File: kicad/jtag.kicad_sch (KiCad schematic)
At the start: 50 parts, among them J3 USB4105-GF-A, J4 Conn_01x02_Male, J5 3220-10-0100-00, U10 NTB0104BQ,115, U13 NTB0104BQ,115, U17 93C56, U2 FT2232HL-REEL, Y2 12MHz

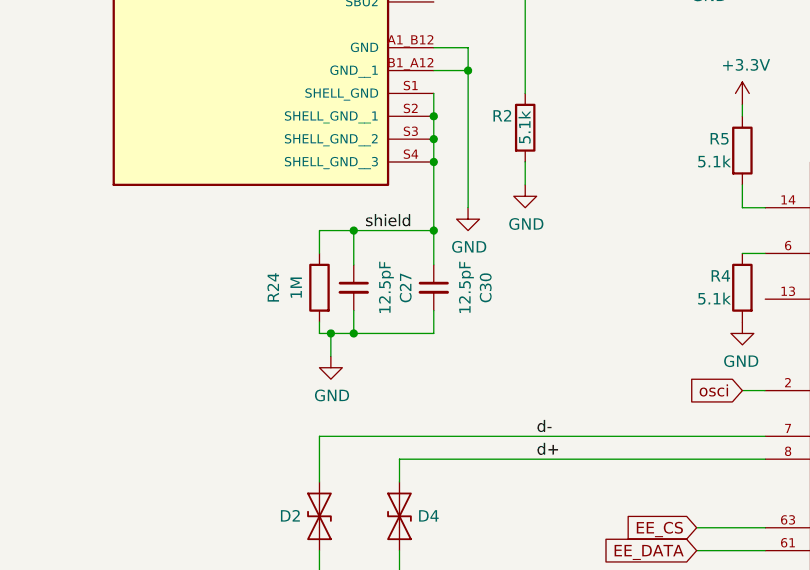
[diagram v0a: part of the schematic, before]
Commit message: directly grounded the USB shield
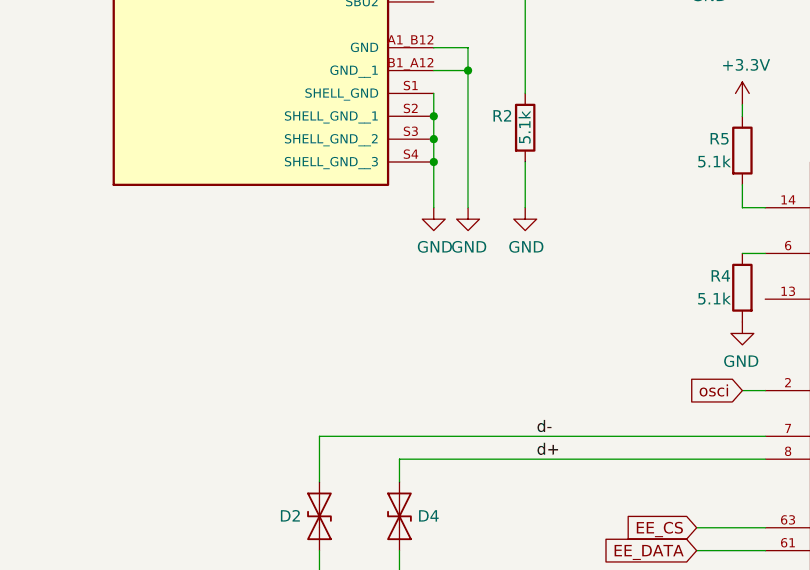
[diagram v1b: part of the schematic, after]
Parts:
- removed C27, C30: 12.5pF, Capacitor_SMD:C_0603_1608Metric, symbol Device:C_Small
- removed R24: 1M, Resistor_SMD:R_0603_1608Metric_Pad0.98x0.95mm_HandSolder, symbol Device:R
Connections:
- net shield is gone; now on net GND: J3.S1 (SHELL_GND), J3.S2 (SHELL_GND__1), J3.S3 (SHELL_GND__2), J3.S4 (SHELL_GND__3)
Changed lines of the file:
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@@
 (kicad_sch (version 20230121) (generator eeschema)
   (paper "A4")
-  (junction (at 62.23 76.2) (diameter 0) (color 0 0 0 0)
-  )
   (junction (at 255.27 67.31) (diameter 0) (color 0 0 0 0)
   )
   (junction (at 250.19 62.23) (diameter 0) (color 0 0 0 0)
   )
-  (junction (at 62.23 64.77) (diameter 0) (color 0 0 0 0)
-  )
   (junction (at 140.97 25.4) (diameter 0) (color 0 0 0 0)
   )
@@
   (junction (at 245.11 115.57) (diameter 0) (color 0 0 0 0)
   )
-  (junction (at 71.12 64.77) (diameter 0) (color 0 0 0 0)
-  )
   (junction (at 166.37 77.47) (diameter 0) (color 0 0 0 0)
   )
@@
   (junction (at 242.57 57.15) (diameter 0) (color 0 0 0 0)
   )
-  (junction (at 59.69 76.2) (diameter 0) (color 0 0 0 0)
-  )
   (junction (at 22.86 185.42) (diameter 0) (color 0 0 0 0)
   )
@@
     (stroke (width 0) (type default))
   )
-  (wire (pts (xy 71.12 68.58) (xy 71.12 64.77))
-    (stroke (width 0) (type default))
-  )
   (wire (pts (xy 200.66 34.29) (xy 190.5 34.29))
     (stroke (width 0) (type default))
@@
     (stroke (width 0) (type default))
   )
-  (wire (pts (xy 59.69 76.2) (xy 59.69 78.74))
+  (wire (pts (xy 71.12 57.15) (xy 71.12 62.23))
     (stroke (width 0) (type default))
   )
@@
     (stroke (width 0) (type default))
   )
-  (wire (pts (xy 71.12 57.15) (xy 71.12 64.77))
-    (stroke (width 0) (type default))
-  )
   (wire (pts (xy 163.83 67.31) (xy 185.42 67.31))
     (stroke (width 0) (type default))
@@
     (stroke (width 0) (type default))
   )
-  (wire (pts (xy 71.12 73.66) (xy 71.12 76.2))
-    (stroke (width 0) (type default))
-  )
   (wire (pts (xy 163.83 62.23) (xy 163.83 64.77))
     (stroke (width 0) (type default))
@@
     (stroke (width 0) (type default))
   )
-  (wire (pts (xy 58.42 67.31) (xy 58.42 64.77))
-    (stroke (width 0) (type default))
-  )
   (wire (pts (xy 158.75 92.71) (xy 185.42 92.71))
     (stroke (width 0) (type default))
@@
     (stroke (width 0) (type default))
   )
-  (wire (pts (xy 62.23 64.77) (xy 71.12 64.77))
-    (stroke (width 0) (type default))
-  )
   (wire (pts (xy 105.41 120.65) (xy 105.41 118.11))
     (stroke (width 0) (type default))
@@
     (stroke (width 0) (type default))
   )
-  (wire (pts (xy 81.28 59.69) (xy 81.28 57.15))
+  (wire (pts (xy 81.28 62.23) (xy 81.28 57.15))
     (stroke (width 0) (type default))
   )
@@
     (stroke (width 0) (type default))
   )
-  (wire (pts (xy 58.42 76.2) (xy 59.69 76.2))
-    (stroke (width 0) (type default))
-  )
   (wire (pts (xy 105.41 50.8) (xy 105.41 52.07))
     (stroke (width 0) (type default))
@@
     (stroke (width 0) (type default))
   )
-  (wire (pts (xy 58.42 74.93) (xy 58.42 76.2))
-    (stroke (width 0) (type default))
-  )
   (wire (pts (xy 212.09 80.01) (xy 214.63 80.01))
     (stroke (width 0) (type default))
@@
     (stroke (width 0) (type default))
   )
-  (wire (pts (xy 58.42 64.77) (xy 62.23 64.77))
-    (stroke (width 0) (type default))
-  )
   (wire (pts (xy 250.19 62.23) (xy 271.78 62.23))
     (stroke (width 0) (type default))
@@
     (stroke (width 0) (type default))
   )
-  (wire (pts (xy 59.69 76.2) (xy 62.23 76.2))
-    (stroke (width 0) (type default))
-  )
   (wire (pts (xy 179.07 25.4) (xy 179.07 87.63))
     (stroke (width 0) (type default))
@@
     (stroke (width 0) (type default))
   )
-  (wire (pts (xy 62.23 73.66) (xy 62.23 76.2))
-    (stroke (width 0) (type default))
-  )
   (wire (pts (xy 71.12 46.99) (xy 74.93 46.99))
     (stroke (width 0) (type default))
@@
     (stroke (width 0) (type default))
   )
-  (wire (pts (xy 62.23 64.77) (xy 62.23 68.58))
-    (stroke (width 0) (type default))
-  )
   (wire (pts (xy 245.11 58.42) (xy 245.11 74.93))
     (stroke (width 0) (type default))
@@
     (stroke (width 0) (type default))
   )
-  (wire (pts (xy 71.12 76.2) (xy 62.23 76.2))
-    (stroke (width 0) (type default))
-  )
   (wire (pts (xy 166.37 72.39) (xy 166.37 60.96))
     (stroke (width 0) (type default))
@@
     (effects (font (size 1.27 1.27)) (justify left bottom))
   )
-  (label "shield" (at 63.5 64.77 0) (fields_autoplaced)
-    (effects (font (size 1.27 1.27)) (justify left bottom))
-  )
   (label "d-" (at 26.67 34.29 0) (fields_autoplaced)
     (effects (font (size 1.27 1.27)) (justify left bottom))
@@
     )
   )
-  (symbol (lib_id "Device:C_Small") (at 62.23 71.12 0) (mirror y) (unit 1)
-    (in_bom yes) (on_board yes) (dnp no)
-    (property "Reference" "C27" (at 68.0466 71.12 90)
-      (effects (font (size 1.27 1.27)))
-    )
-    (property "Value" "12.5pF" (at 65.7352 71.12 90)
-      (effects (font (size 1.27 1.27)))
-    )
-    (property "Footprint" "Capacitor_SMD:C_0603_1608Metric" (at 62.23 71.12 0)
-      (effects (font (size 1.27 1.27)) hide)
-    )
-    (property "Datasheet" "~" (at 62.23 71.12 0)
-      (effects (font (size 1.27 1.27)) hide)
-    )
-    (pin "1")
-    (pin "2")
-    (instances
-      (project "OpenHW DevKit"
-        (path "/b0906e10-2fbc-4309-a8b4-6fc4cd1a5490/05c5e7d7-6e8b-47d0-a3ba-1eadff858466"
-          (reference "C27") (unit 1)
-        )
-      )
-    )
-  )
   (symbol (lib_id "Diode:ESD9B5.0ST5G") (at 67.31 96.52 270) (unit 1)
     (in_bom yes) (on_board yes) (dnp no)
@@
     )
   )
-  (symbol (lib_id "power:GND") (at 59.69 78.74 0) (unit 1)
+  (symbol (lib_id "power:GND") (at 71.12 62.23 0) (unit 1)
     (in_bom yes) (on_board yes) (dnp no)
-    (property "Reference" "#PWR010" (at 59.69 85.09 0)
+    (property "Reference" "#PWR010" (at 71.12 68.58 0)
       (effects (font (size 1.27 1.27)) hide)
     )
-    (property "Value" "GND" (at 59.817 83.1342 0)
+    (property "Value" "GND" (at 71.247 66.6242 0)
       (effects (font (size 1.27 1.27)))
     )
-    (property "Footprint" "" (at 59.69 78.74 0)
+    (property "Footprint" "" (at 71.12 62.23 0)
       (effects (font (size 1.27 1.27)) hide)
     )
-    (property "Datasheet" "" (at 59.69 78.74 0)
+    (property "Datasheet" "" (at 71.12 62.23 0)
       (effects (font (size 1.27 1.27)) hide)
     )
@@
     )
   )
-  (symbol (lib_id "power:GND") (at 81.28 59.69 0) (unit 1)
+  (symbol (lib_id "power:GND") (at 81.28 62.23 0) (unit 1)
     (in_bom yes) (on_board yes) (dnp no)
-    (property "Reference" "#PWR017" (at 81.28 66.04 0)
+    (property "Reference" "#PWR017" (at 81.28 68.58 0)
       (effects (font (size 1.27 1.27)) hide)
     )
-    (property "Value" "GND" (at 81.407 64.0842 0)
+    (property "Value" "GND" (at 81.407 66.6242 0)
       (effects (font (size 1.27 1.27)))
     )
-    (property "Footprint" "" (at 81.28 59.69 0)
+    (property "Footprint" "" (at 81.28 62.23 0)
       (effects (font (size 1.27 1.27)) hide)
     )
-    (property "Datasheet" "" (at 81.28 59.69 0)
+    (property "Datasheet" "" (at 81.28 62.23 0)
       (effects (font (size 1.27 1.27)) hide)
     )
@@
     )
   )
-  (symbol (lib_id "Device:C_Small") (at 71.12 71.12 0) (unit 1)
-    (in_bom yes) (on_board yes) (dnp no)
-    (property "Reference" "C30" (at 76.9366 71.12 90)
-      (effects (font (size 1.27 1.27)))
-    )
-    (property "Value" "12.5pF" (at 74.6252 71.12 90)
-      (effects (font (size 1.27 1.27)))
-    )
-    (property "Footprint" "Capacitor_SMD:C_0603_1608Metric" (at 71.12 71.12 0)
-      (effects (font (size 1.27 1.27)) hide)
-    )
-    (property "Datasheet" "~" (at 71.12 71.12 0)
-      (effects (font (size 1.27 1.27)) hide)
-    )
-    (pin "1")
-    (pin "2")
-    (instances
-      (project "OpenHW DevKit"
-        (path "/b0906e10-2fbc-4309-a8b4-6fc4cd1a5490/05c5e7d7-6e8b-47d0-a3ba-1eadff858466"
-          (reference "C30") (unit 1)
-        )
-      )
-    )
-  )
   (symbol (lib_id "Device:C_Small") (at 255.27 25.4 0) (mirror y) (unit 1)
     (in_bom yes) (on_board yes) (dnp no)
@@
         )
       )
-    )
-  )
-  (symbol (lib_id "Device:R") (at 58.42 71.12 0) (mirror y) (unit 1)
-    (in_bom yes) (on_board yes) (dnp no)
-    (property "Reference" "R24" (at 53.34 71.12 90)
-      (effects (font (size 1.27 1.27)))
-    )
-    (property "Value" "1M" (at 55.88 71.12 90)
-      (effects (font (size 1.27 1.27)))
-    )
-    (property "Footprint" "Resistor_SMD:R_0603_1608Metric_Pad0.98x0.95mm_HandSolder" (at 60.198 71.12 90)
-      (effects (font (size 1.27 1.27)) hide)
-    )
-    (property "Datasheet" "~" (at 58.42 71.12 0)
-      (effects (font (size 1.27 1.27)) hide)
-    )
-    (pin "1")
-    (pin "2")
-    (instances
-      (project "OpenHW DevKit"
-        (path "/b0906e10-2fbc-4309-a8b4-6fc4cd1a5490/05c5e7d7-6e8b-47d0-a3ba-1eadff858466"
-          (reference "R24") (unit 1)
-        )
-      )
